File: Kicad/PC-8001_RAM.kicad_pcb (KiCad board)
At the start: 2 copper layers, 47 x 91 mm, 16 parts, among them J1 PC-8001 BUS, J2 PC-8001 BUS, U1 GAL22V10, U2 62256, U3 CY7C199

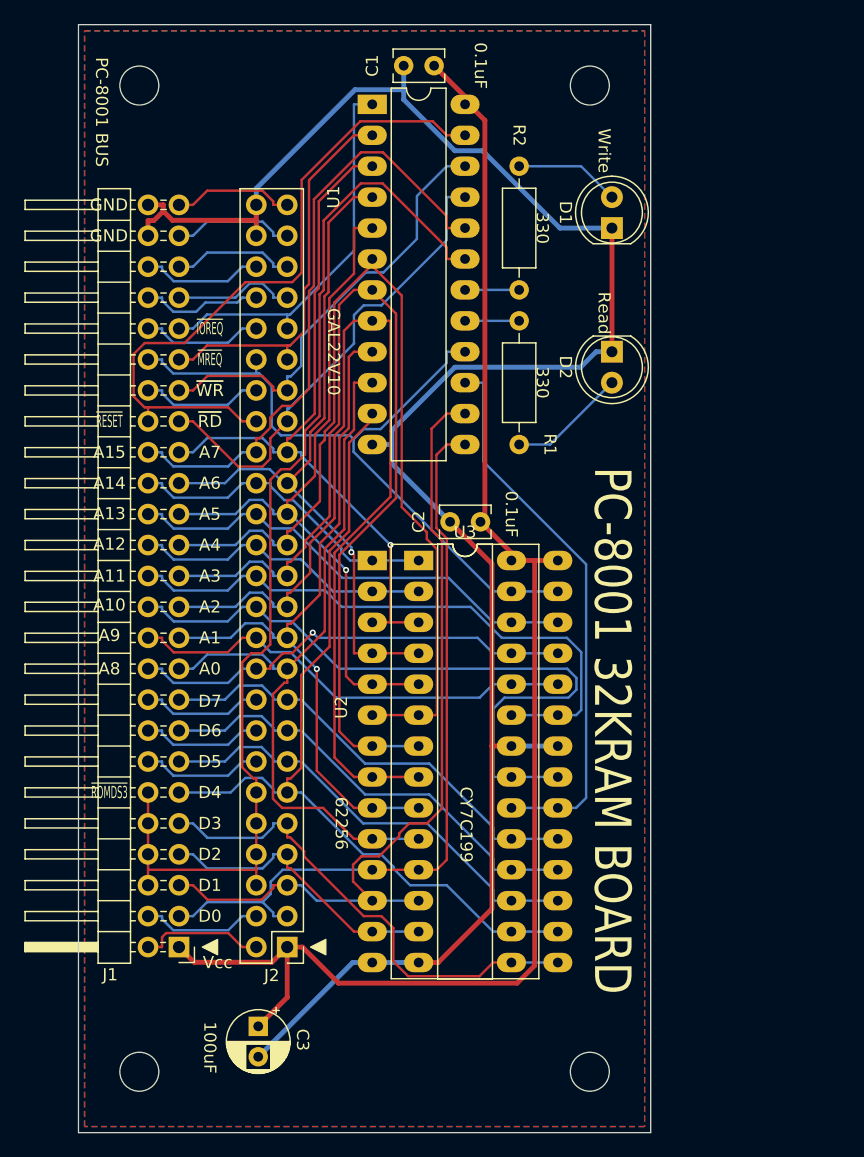
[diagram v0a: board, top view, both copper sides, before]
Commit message: Add files via upload
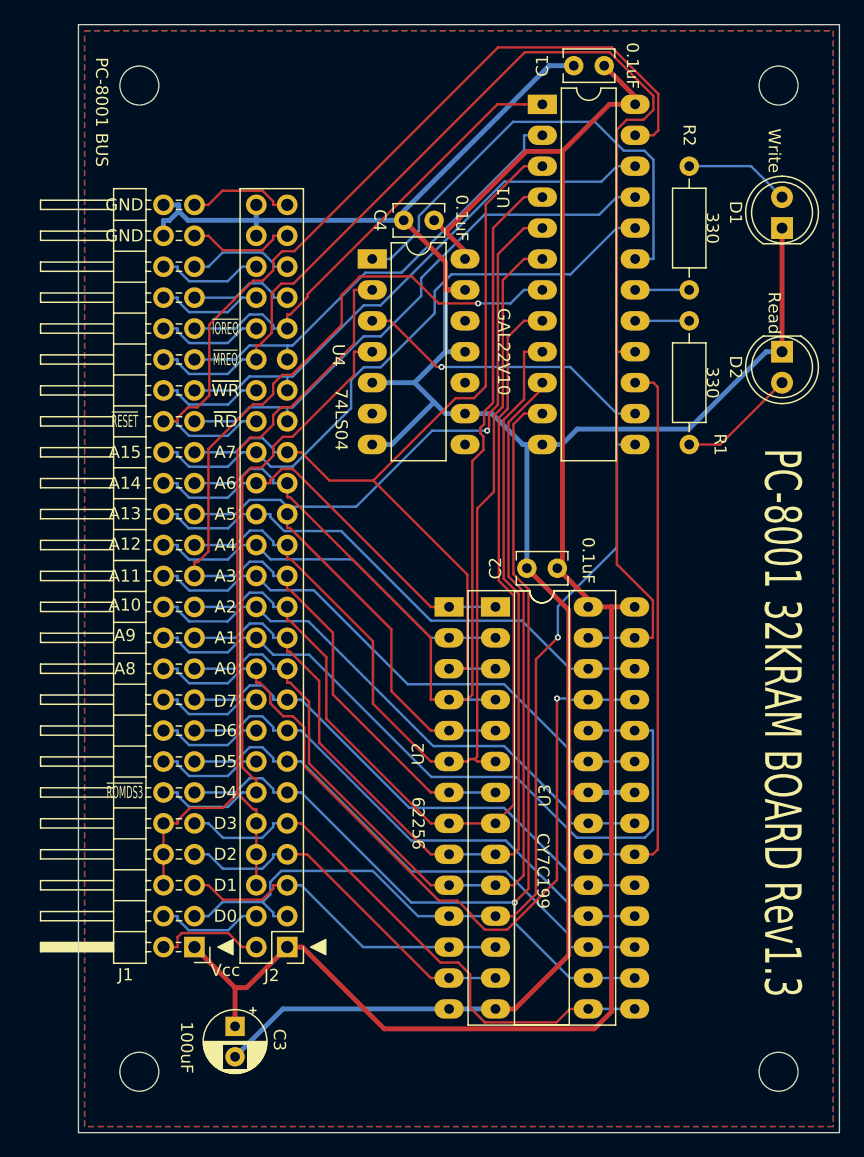
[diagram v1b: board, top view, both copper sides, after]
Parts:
- added C4: 0.1uF, Capacitor_THT:C_Rect_L4.0mm_W2.5mm_P2.50mm, F.Cu at (116.8, 80.0)
- added U4: 74LS04, Package_DIP:DIP-14_W7.62mm_LongPads, F.Cu at (111.8, 83.2)
- moved MH2 15.5 mm to (145.1, 149.9)
- moved MH3 15.5 mm to (145.1, 68.9)
- moved C1 14.0 mm to (130.8, 67.3)
- moved D1 14.0 mm to (145.4, 80.6)
- moved D2 14.0 mm to (145.4, 90.8)
- moved U1 14.0 mm to (125.7, 70.5)
- moved R1 14.0 mm to (137.8, 88.3)
- moved R2 14.0 mm to (137.8, 85.7)
- moved U3 7.37 mm to (121.9, 111.8)
- moved U2 7.37 mm to (118.1, 111.8)
- moved C2 7.37 mm to (127.0, 108.6)
- moved C3 1.91 mm to (100.5, 146.2)
- moved J1 1.27 mm to (97.2, 139.7)
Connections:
- J1 pad 12: /~ROMDS0 -> /~ROMDS3
- J2 pad 12: /~ROMDS0 -> /~ROMDS3
- U1 pad 14: /D1 -> Net-(U1-Pad14)
- U1 pad 19: /~ROMDS0 -> Net-(U1-Pad19)
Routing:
- net /~WE: track 58.0 -> 110.5 mm
- net /~ROMDS3: track 0.00 -> 51.8 mm
- net /D1: track 69.1 -> 28.0 mm
- net GND: track 161.0 -> 201.4 mm
- net Net-(U1-Pad19): track 0.00 -> 39.4 mm
- net /A8: track 36.8 -> 68.4 mm
- net +5V: track 120.5 -> 147.6 mm
- net Net-(U1-Pad14): track 0.00 -> 24.7 mm, vias 0 -> 1
- net /A6: track 58.7 -> 83.3 mm, vias 1 -> 0
- net /A9: track 37.3 -> 61.8 mm
- net /A1: track 59.0 -> 82.5 mm, vias 1 -> 0
- net /~ROMDS0: track 91.4 -> 68.4 mm
- net /A0: track 61.9 -> 81.6 mm
- net /~RESET: track 55.6 -> 72.8 mm
- net /A5: track 59.2 -> 75.5 mm
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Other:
- board size 47 x 91 mm -> 62.5 x 91 mm
- board text added: "74LS04"
- board text added: "PC-8001 32KRAM BOARD Rev1.3"
- board text removed: "PC-8001 32KRAM BOARD"
